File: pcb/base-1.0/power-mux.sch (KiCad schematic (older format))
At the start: 23 parts, among them Q201 IRF7324TRPBF, Q202 IRF7324TRPBF, Q203 IRF7324TRPBF, U201 LTC4417

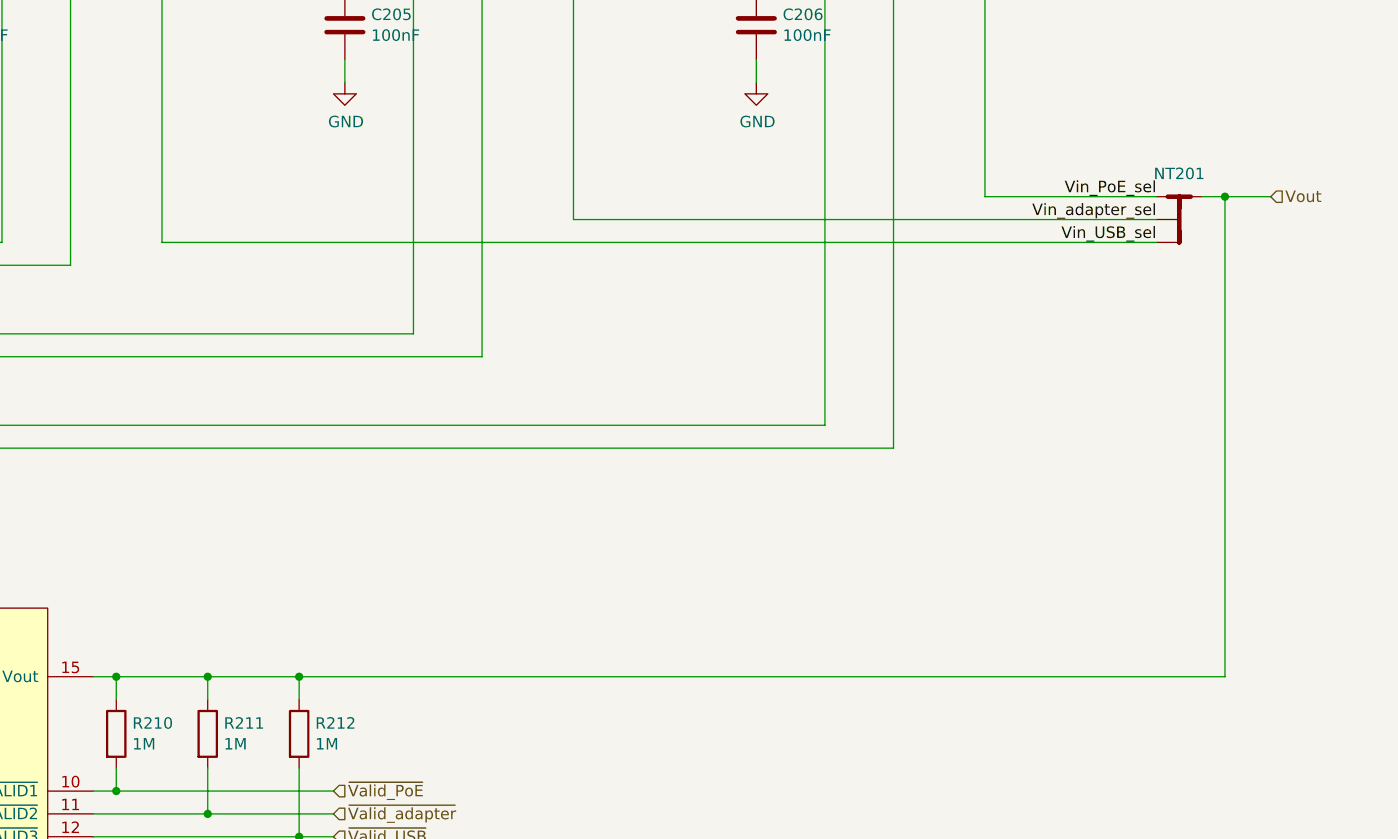
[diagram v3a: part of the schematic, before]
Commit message: o More PCB work.
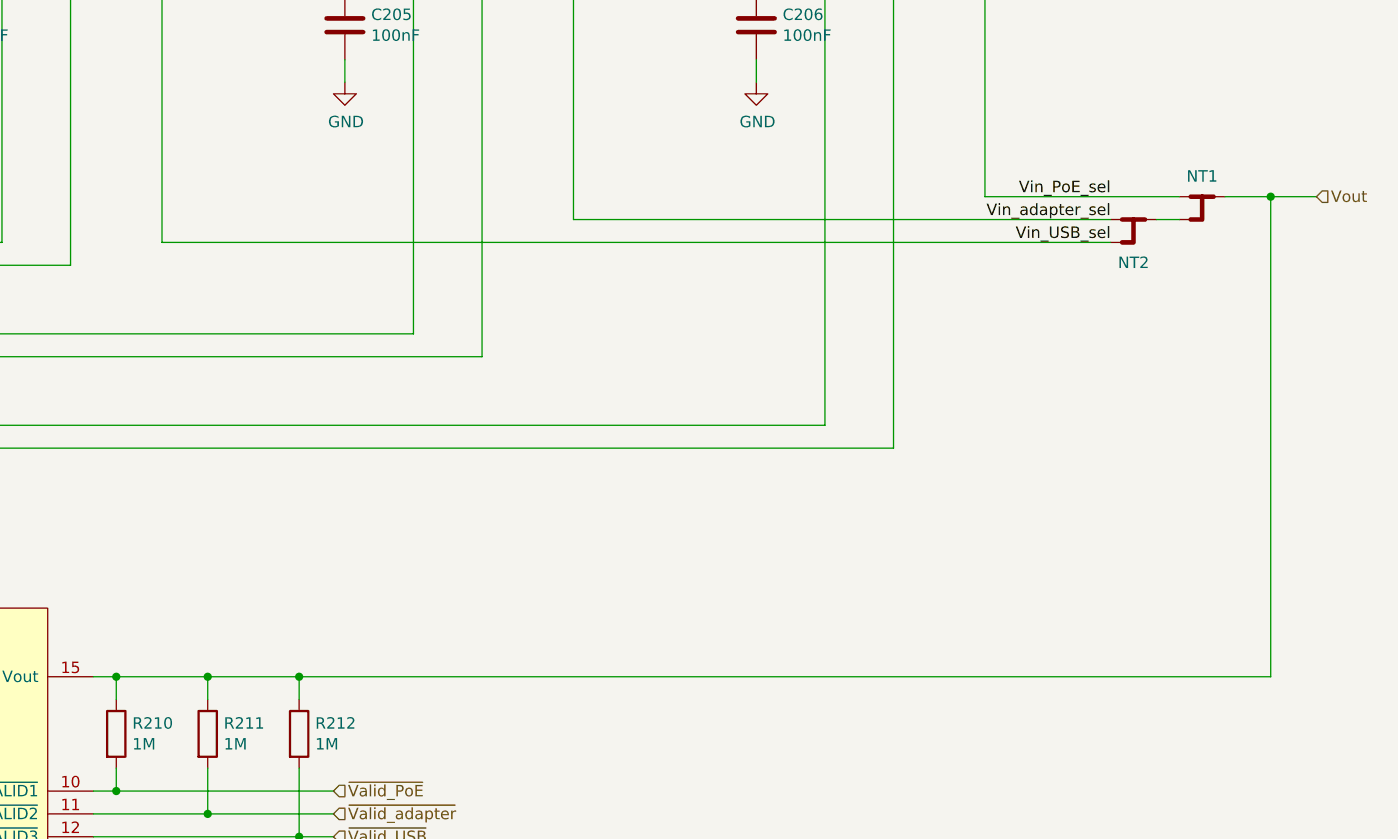
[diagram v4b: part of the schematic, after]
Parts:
- removed NT201: Net-Tie_3_to_1, NetTie:NetTie-4_SMD_Pad0.5mm, symbol unlockoslo:Net-Tie_3_to_1
- added NT1, NT2: Net-Tie_3, UnlockOslo:NetTie-3_SMD_Pad0.5mm_132, symbol Device:Net-Tie_3
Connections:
- net Vin_PoE_sel: now also NT1.1
- net Vin_USB_sel: now also NT2.3
- net Vin_adapter_sel: now also NT2.1
- net Vout: now also NT1.2
- new net: NT1.3, NT2.2
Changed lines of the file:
@@
 TODO:\n* Calculate resistor values
 Wire Wire Line
-	6500 5500 10550 5500
+	6500 5500 10750 5500
 Connection ~ 5900 1900
 Wire Wire Line
@@
 Wire Wire Line
 	9300 1800 9500 1800
-Wire Wire Line
-	9500 3400 10250 3400
 Wire Wire Line
 	9500 1900 9500 3400
@@
 Text HLabel 1100 800  0    50   Input ~ 0
 Vin_PoE
-Text HLabel 10750 3400 2    50   Input ~ 0
+Text HLabel 10950 3400 2    50   Input ~ 0
 Vout
 Wire Wire Line
-	10550 3400 10750 3400
-Connection ~ 10550 3400
-Wire Wire Line
-	10450 3400 10550 3400
-$Comp
-L unlockoslo:Net-Tie_3_to_1 NT201
-U 1 1 5D02029B
-P 10350 3400
-F 0 "NT201" H 10350 3500 50  0000 C CNN
-F 1 "Net-Tie_3_to_1" H 10350 3490 50  0001 C CNN
-F 2 "NetTie:NetTie-4_SMD_Pad0.5mm" H 10350 3400 50  0001 C CNN
-F 3 "~" H 10350 3400 50  0001 C CNN
-	1    10350 3400
-	1    0    0    -1
-$EndComp
-Wire Wire Line
-	10550 5500 10550 3400
+	10750 3400 10950 3400
+Connection ~ 10750 3400
+Wire Wire Line
+	10750 5500 10750 3400
 Connection ~ 1400 2200
 Wire Wire Line
@@
 	4600 5000 4600 4100
 Wire Wire Line
-	7700 3500 10250 3500
-Wire Wire Line
-	5900 3600 10250 3600
+	7700 3500 10050 3500
+Wire Wire Line
+	5900 3600 10050 3600
 Wire Wire Line
 	7700 1900 7700 3500
@@
 Wire Wire Line
 	5100 1900 5200 1900
-Text Label 10250 3600 2    50   ~ 0
+Text Label 10050 3600 2    50   ~ 0
 Vin_USB_sel
-Text Label 10250 3500 2    50   ~ 0
+Text Label 10050 3500 2    50   ~ 0
 Vin_adapter_sel
-Text Label 10250 3400 2    50   ~ 0
+Text Label 10050 3400 2    50   ~ 0
 Vin_PoE_sel
+$Comp
+L Device:Net-Tie_3 NT2
+U 1 1 5D13BBF9
+P 10150 3500
+F 0 "NT2" H 10150 3311 50  0000 C CNN
+F 1 "Net-Tie_3" H 10150 3590 50  0001 C CNN
+F 2 "UnlockOslo:NetTie-3_SMD_Pad0.5mm_132" H 10150 3500 50  0001 C CNN
+F 3 "~" H 10150 3500 50  0001 C CNN
+	1    10150 3500
+	1    0    0    -1
+$EndComp
+$Comp
+L Device:Net-Tie_3 NT1
+U 1 1 5D13CB32
+P 10450 3400
+F 0 "NT1" H 10450 3489 50  0000 C CNN
+F 1 "Net-Tie_3" H 10450 3490 50  0001 C CNN
+F 2 "UnlockOslo:NetTie-3_SMD_Pad0.5mm_132" H 10450 3400 50  0001 C CNN
+F 3 "~" H 10450 3400 50  0001 C CNN
+	1    10450 3400
+	1    0    0    -1
+$EndComp
+Wire Wire Line
+	10550 3400 10750 3400
+Wire Wire Line
+	9500 3400 10350 3400
+Wire Wire Line
+	10250 3500 10350 3500
 $EndSCHEMATC
